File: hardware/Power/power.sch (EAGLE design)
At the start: 44 parts, among them IC10 ACS712ELCTR-05B-T, IC20 LM358_SOIC, K1 SSR, Q1 PNP, T20 ZMPT101B, U4 PC817XI, X1 057-006-1

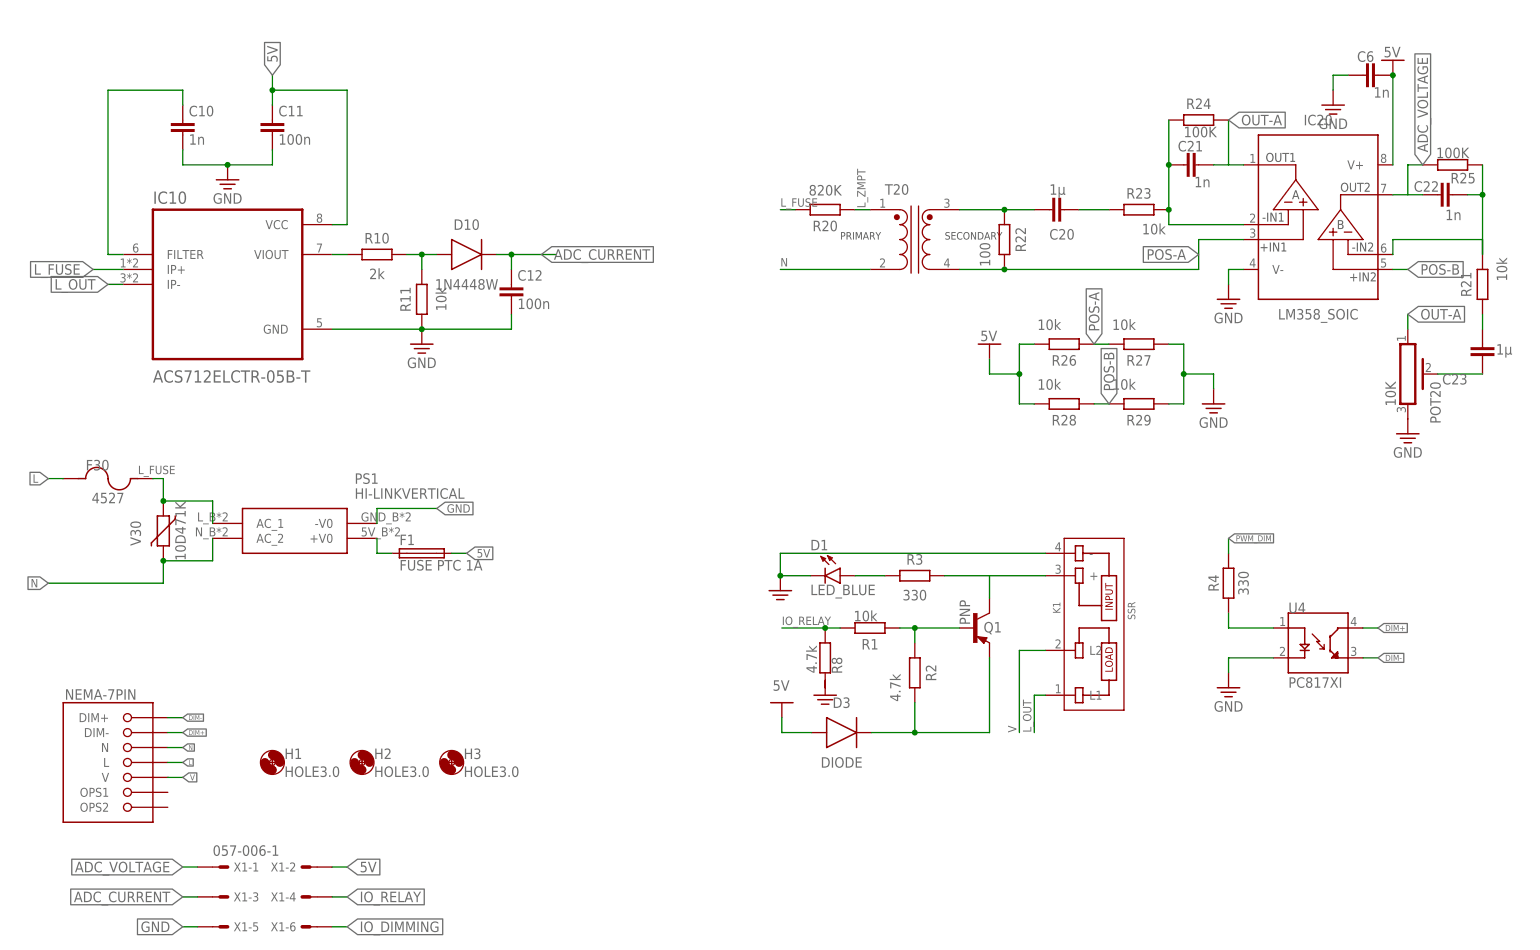
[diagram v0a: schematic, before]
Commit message: bakcup before ganti ukuran smd
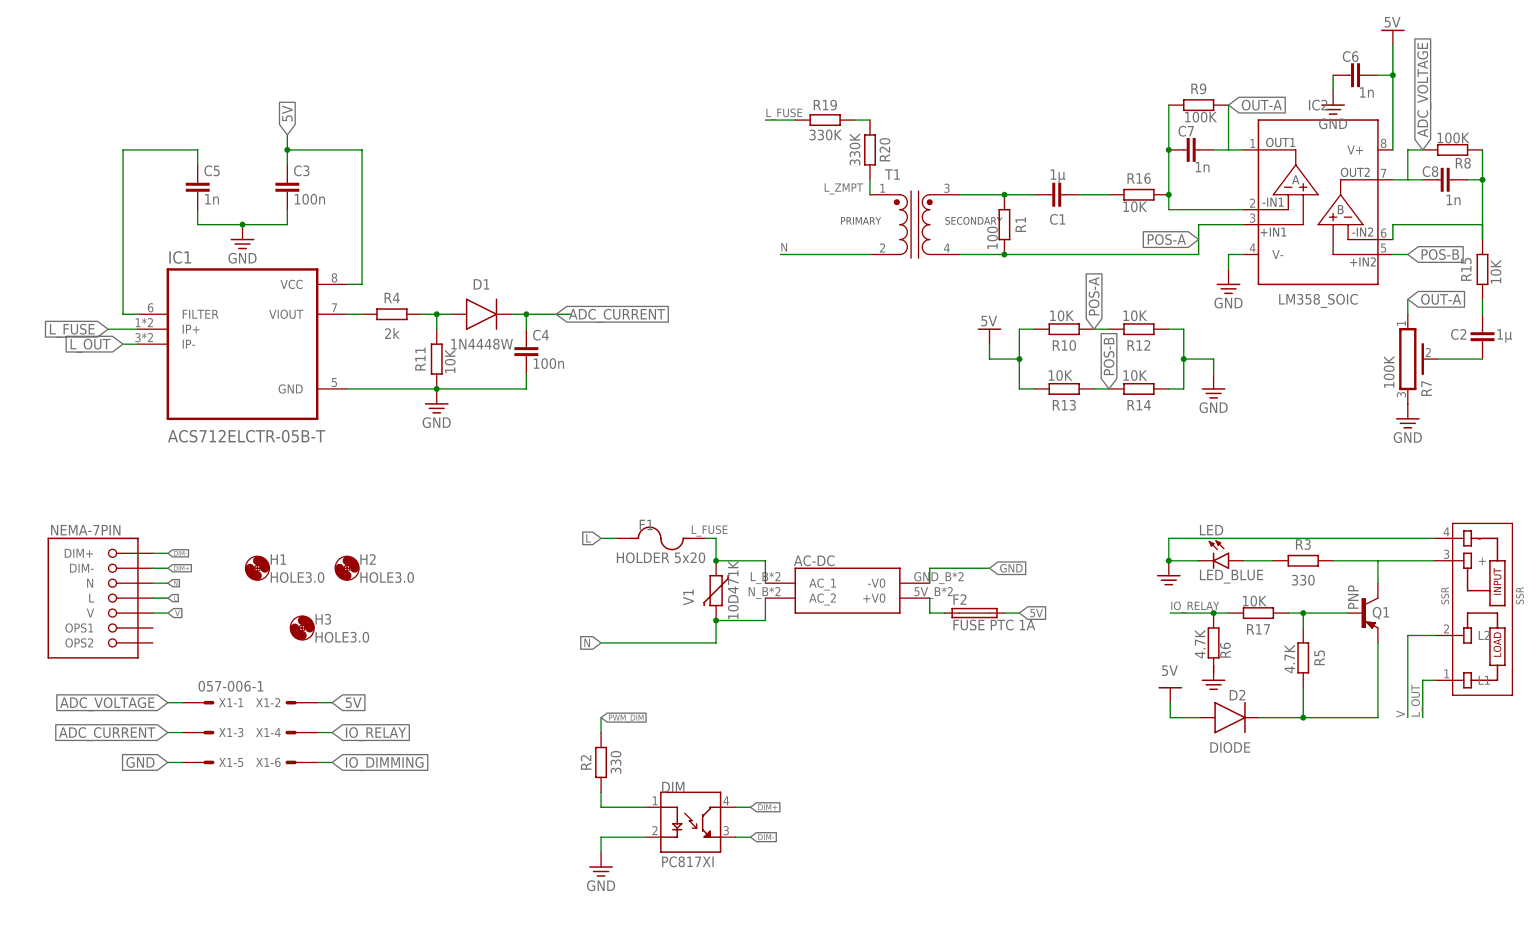
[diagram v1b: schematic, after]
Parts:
- removed C10, C21, C22: 1n, Capacitor:C_CHIP-0603(1608-METRIC)
- removed C11, C12: 100n, Capacitor:C_CHIP-0603(1608-METRIC)
- removed C20, C23: 1µ, Capacitor:C_CHIP-0603(1608-METRIC)
- removed D10: 1N4448W, Diode:DIODE_1N4148W-7-F_SOD123G
- removed D3: DIODE, Diode:DIODEDO-214AC(SMA)
- removed F30: 4527, Fuse Holder:4527
- removed IC10: ACS712ELCTR-05B-T, XLKM#4:ACS712ELCTR-05B-T
- removed IC20: LM358_SOIC, IC_Linear:LM358_SOIC
- removed K1: SSR, XLKM#4:SSR
- removed POT20: 10K, Resistor:PV36W
- removed PS1: HI-LINKVERTICAL, XLKM#4:HI-LINKVERTICAL
- removed R21, R23, R26, R27, R28, R29: 10k, Resistor:R_CHIP-0603(1608-METRIC)
- removed R22: 100, rcl:R-EU_R1206
- removed R24, R25: 100K, Resistor:R_CHIP-0603(1608-METRIC)
- removed T20: ZMPT101B, XLKM#4:ZMPT101B
- removed U4: PC817XI, SnapEDA Library:PC817XI
- removed V30: 10D471K, XLKM#4:VARISTOR
- added AC-DC: HI-LINKVERTICAL, XLKM#4:HI-LINKVERTICAL
- added C1, C2: 1µ, Capacitor:C_CHIP-0603(1608-METRIC)
- added C3, C4: 100n, Capacitor:C_CHIP-0603(1608-METRIC)
- added C5, C7, C8: 1n, Capacitor:C_CHIP-0603(1608-METRIC)
- added D2: DIODE, Diode:DIODEDO-214AC(SMA)
- added DIM: PC817XI, SnapEDA Library:PC817XI
- added F2: FUSE PTC 1A, Circuit-Protection:FUSE_CHIP-1206(3216-METRIC)
- added IC1: ACS712ELCTR-05B-T, XLKM#4:ACS712ELCTR-05B-T
- added IC2: LM358_SOIC, IC_Linear:LM358_SOIC
- added LED: LED_BLUE, LED:CHIP-FLAT-B_0603-0.55MM
- added R12, R13, R14, R15, R16, R17: 10K, Resistor:R_CHIP-0603(1608-METRIC)
- added R19: 330K, Resistor:R_AXIAL-7.2MM-PITCH
- added R5, R6: 4.7K, Resistor:R_CHIP-0603(1608-METRIC)
- added R7: 100K, Resistor:PV36W
- added R9: 100K, Resistor:R_CHIP-0603(1608-METRIC)
- added SSR: SSR, XLKM#4:SSR
- added T1: ZMPT101B, XLKM#4:ZMPT101B
- added V1: 10D471K, XLKM#4:VARISTOR
- D1: value LED_BLUE -> 1N4448W; device LED:CHIP-FLAT-B_0603-0.55MM -> Diode:DIODE_1N4148W-7-F_SOD123G
- F1: value FUSE PTC 1A -> HOLDER 5x20; device Circuit-Protection:FUSE_CHIP-1206(3216-METRIC) -> Fuse Holder:4527
- R1: value 10k -> 100; device Resistor:R_CHIP-0603(1608-METRIC) -> rcl:R-EU_R1206
- R10: value 2k -> 10K
- R11: value 10k -> 10K
- R2: value 4.7k -> 330
- R20: value 820K -> 330K; device rcl:R-EU_R0805 -> Resistor:R_AXIAL-7.2MM-PITCH
- R4: value 330 -> 2k
- R8: value 4.7k -> 100K
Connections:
- new net N$5: R19.2, R20.1
- net 5V: now also C3.1, D2.A, F2.2, IC1.VCC, IC2.V+, R10.2, R13.2; no longer C11.1, D3.A, F1.2, IC10.VCC, IC20.V+, R26.2, R28.2
- net ADC_CURRENT: now also C4.1, D1.C; no longer C12.1, D10.C
- net ADC_VOLTAGE: now also R8.2; no longer R25.2
- net DIM+: now also DIM.CT; no longer U4.CT
- net DIM-: now also DIM.ET; no longer U4.ET
- net GND: now also AC-DC.-V0, C3.2, C4.2, C5.2, DIM.C, IC1.GND, IC2.V-, LED.C, R12.1, R14.1, R7.P$3, SSR.-; no longer C10.2, C11.2, C12.2, D1.C, IC10.GND, IC20.V-, K1.-, POT20.P$3, PS1.-V0, R27.1, R29.1, U4.C
- net IO_RELAY: now also R17.2, R6.1; no longer R1.2, R8.1
- net L: now also F1.1; no longer F30.1
- net L_FUSE: now also AC-DC.AC_1, F1.2, IC1.IP+, R19.1, V1.1; no longer F30.2, IC10.IP+, PS1.AC_1, R20.2, V30.1
- net L_OUT: now also IC1.IP-, SSR.L1; no longer IC10.IP-, K1.L1
- net L_ZMPT: now also R20.2, T1.1; no longer R20.1, T20.1
- net N: now also AC-DC.AC_2, T1.2, V1.2; no longer PS1.AC_2, T20.2, V30.2
- net N$1: now also C1.1, R1.1, T1.3; no longer C20.1, R22.1, T20.3
- net N$11: now also C5.1, IC1.FILTER; no longer C10.1, IC10.FILTER
- net N$12: now also D2.C, R5.2; no longer D3.C, R2.2
- net N$13: now also R17.1, R5.1; no longer R1.1, R2.1
- net N$15: now also SSR.+; no longer K1.+
- net N$16: now also C8.2, IC2.-IN2, R15.2, R8.1; no longer C22.2, IC20.-IN2, R21.2, R25.1
- net N$17: now also C2.2, R15.1; no longer C23.2, R21.1
- net N$18: now also C2.1, R7.P$2; no longer C23.1, POT20.P$2
- net N$2: now also C7.2, IC2.OUT1; no longer C21.2, IC20.OUT1
- net N$22: now also AC-DC.+V0, F2.1; no longer F1.1, PS1.+V0
- net N$24: now also LED.A; no longer D1.A
- net N$27: now also DIM.A, R2.1; no longer R4.1, U4.A
- net N$3: now also C1.2, R16.1; no longer C20.2, R23.1
- net N$4: now also IC1.VIOUT, R4.1; no longer IC10.VIOUT, R10.1
- net N$7: now also C8.1, IC2.OUT2; no longer C22.1, IC20.OUT2
- net N$8: now also C7.1, IC2.-IN1, R16.2, R9.1; no longer C21.1, IC20.-IN1, R23.2, R24.1
- net N$9: now also D1.A, R4.2; no longer D10.A, R10.2
- net OUT-A: now also R7.P$1, R9.2; no longer POT20.P$1, R24.2
- net POS-A: now also IC2.+IN1, R1.2, R10.1, R12.2, T1.4; no longer IC20.+IN1, R22.2, R26.1, R27.2, T20.4
- net POS-B: now also IC2.+IN2, R13.1, R14.2; no longer IC20.+IN2, R28.1, R29.2
- net PWM_DIM: now also R2.2; no longer R4.2
- net V: now also SSR.L2; no longer K1.L2
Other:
- moved on the sheet: C6, H1, H2, H3, NEMA-7PIN, Q1, R1, R10, R11, R2, R20, R3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
